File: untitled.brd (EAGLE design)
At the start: 18.4 x 16.2 mm, 13 parts, among them IC1 NE555D

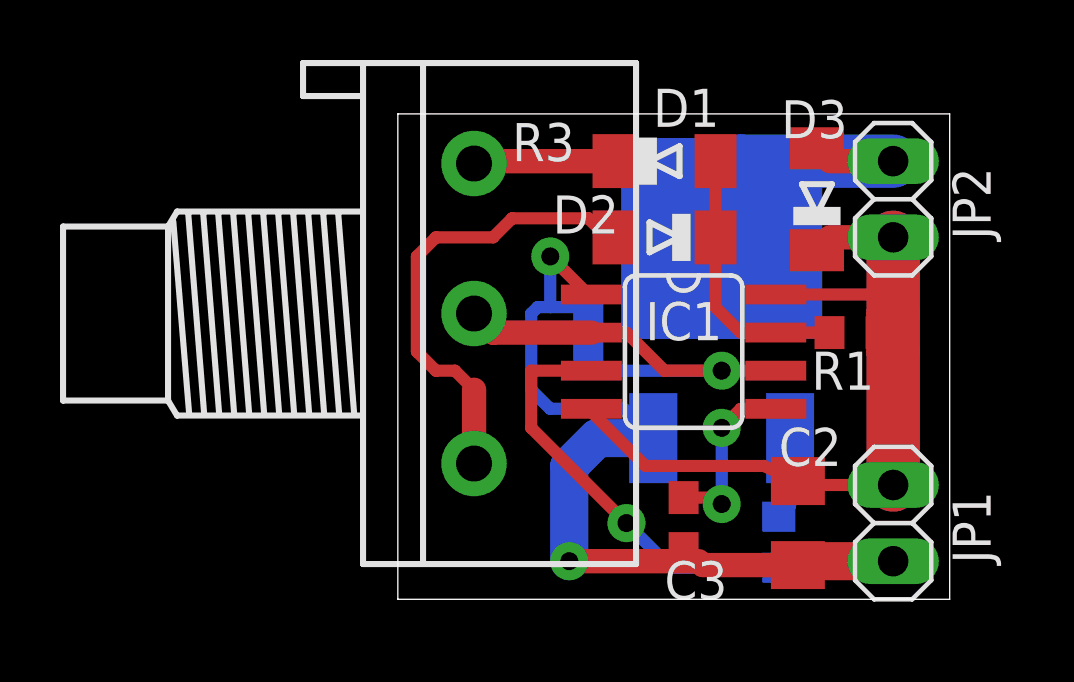
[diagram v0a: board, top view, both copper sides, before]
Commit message: Prepared for prodution
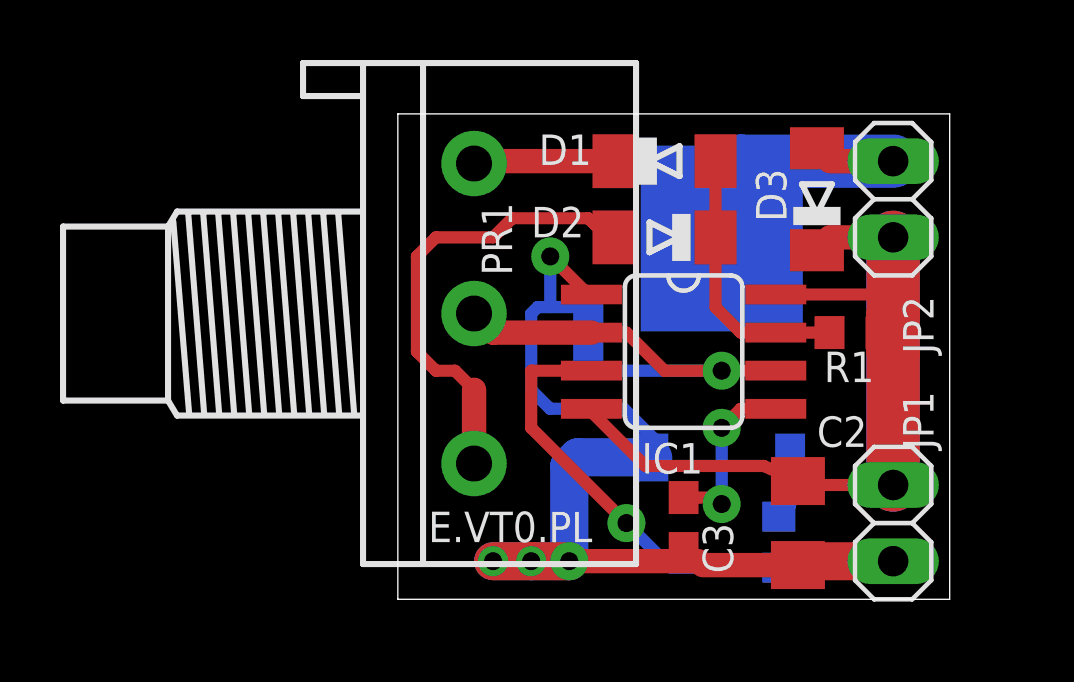
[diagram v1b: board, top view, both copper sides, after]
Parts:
- PR1: value (none) -> 10K
- Q1: value (none) -> MOSFET-N; device IGBT:TO252_STM -> mosfet_to252:TO252
- renumbered R3 to PR1
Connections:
- net GND: now also Q1.2; no longer Q1.3
- net N$11: now also Q1.3; no longer Q1.2
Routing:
- net GND: track 31.0 -> 36.4 mm, vias 2 -> 4
- net N$7: track 2.77 -> 2.13 mm
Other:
- board text added: "+"
- board text added: "-"
- board text added: "2018"
- board text added: "E.VT0.PL"
- board text added: "OUT"
- board text added: "VIN"

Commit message: Description update
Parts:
- D1, D2, D3: value (none) -> LL4148
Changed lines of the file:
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@@
 <attribute name="NAME" x="25.908" y="6.096" size="1.016" layer="25" font="vector" ratio="11"/>
 </element>
-<element name="D1" library="diode" package="MINIMELF" value="" x="26.67" y="16.51" smashed="yes">
+<element name="D1" library="diode" package="MINIMELF" value="LL4148" x="26.67" y="16.51" smashed="yes">
 <attribute name="NAME" x="22.479" y="16.383" size="1.016" layer="25" font="vector" ratio="11"/>
 <attribute name="VALUE" x="25.019" y="14.097" size="1.27" layer="27"/>
 </element>
-<element name="D2" library="diode" package="MINIMELF" value="" x="26.67" y="13.97" smashed="yes" rot="R180">
+<element name="D2" library="diode" package="MINIMELF" value="LL4148" x="26.67" y="13.97" smashed="yes" rot="R180">
 <attribute name="NAME" x="22.225" y="13.97" size="1.016" layer="25" font="vector" ratio="11"/>
 <attribute name="VALUE" x="28.321" y="16.383" size="1.27" layer="27" rot="R180"/>
@@
 <attribute name="VALUE" x="37.465" y="12.7" size="1.27" layer="27" rot="R90"/>
 </element>
-<element name="D3" library="diode" package="MINIMELF" value="" x="31.75" y="15.24" smashed="yes" rot="R90">
+<element name="D3" library="diode" package="MINIMELF" value="LL4148" x="31.75" y="15.24" smashed="yes" rot="R90">
 <attribute name="NAME" x="29.718" y="16.256" size="1.016" layer="25" font="vector" ratio="11" rot="R270"/>
 <attribute name="VALUE" x="34.163" y="13.589" size="1.27" layer="27" rot="R90"/>
